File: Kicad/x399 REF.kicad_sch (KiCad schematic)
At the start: 75 parts, among them J1 +15V, J2 10Vref, Q1 MMBT3904, Q2 2SD882, Q3 AON7410, U1 LM399, U2 OP07

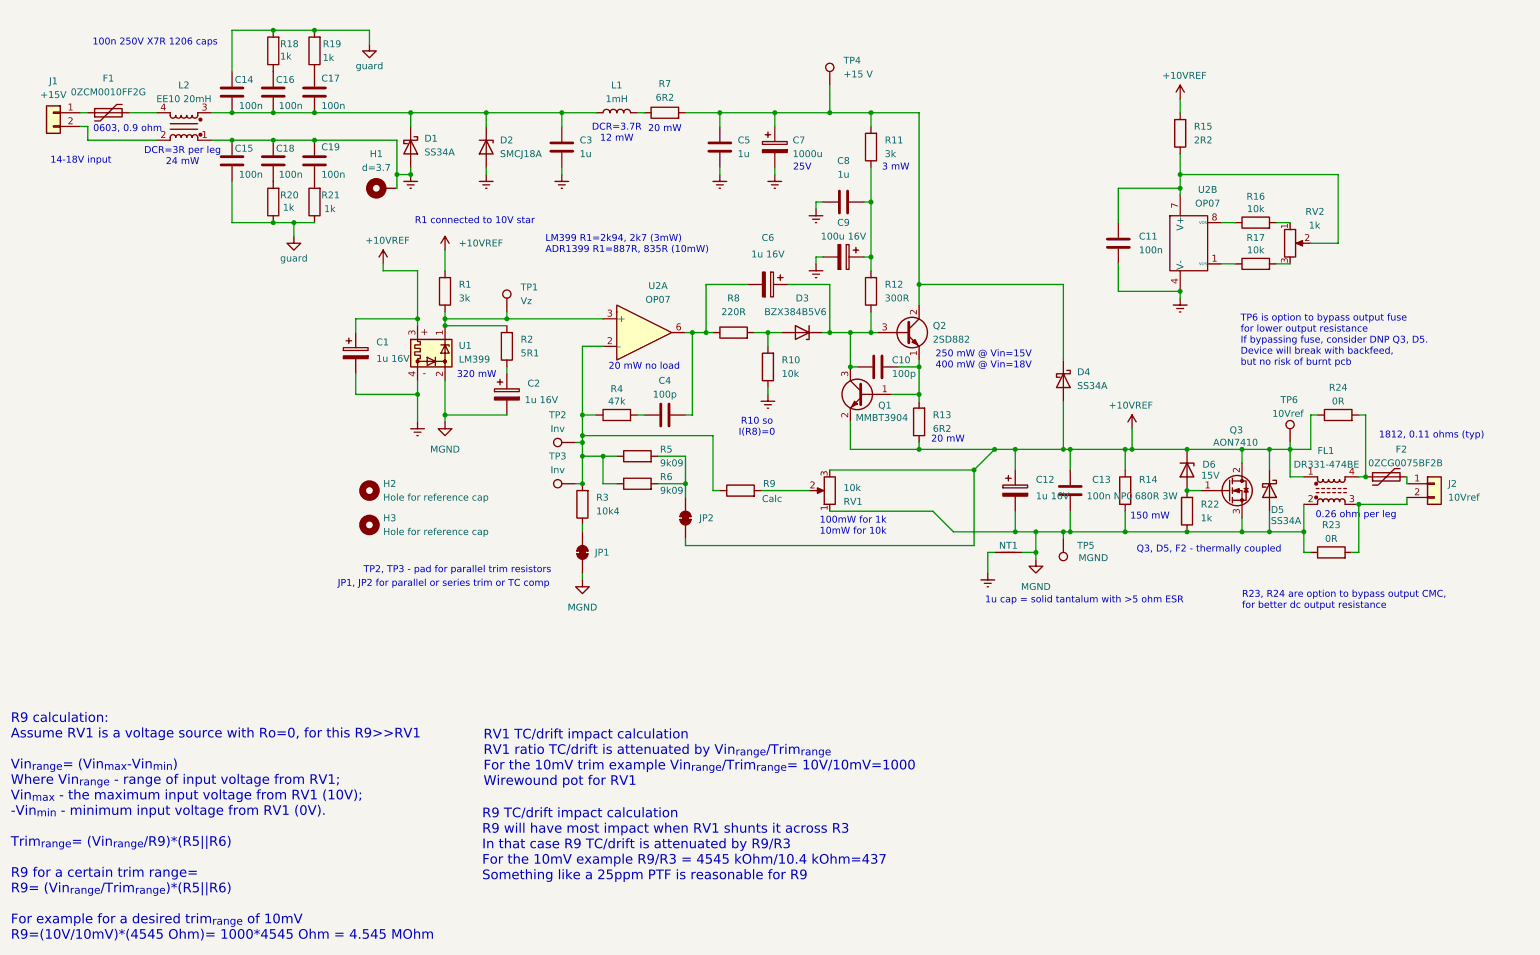
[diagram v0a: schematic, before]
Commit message: Add files via upload
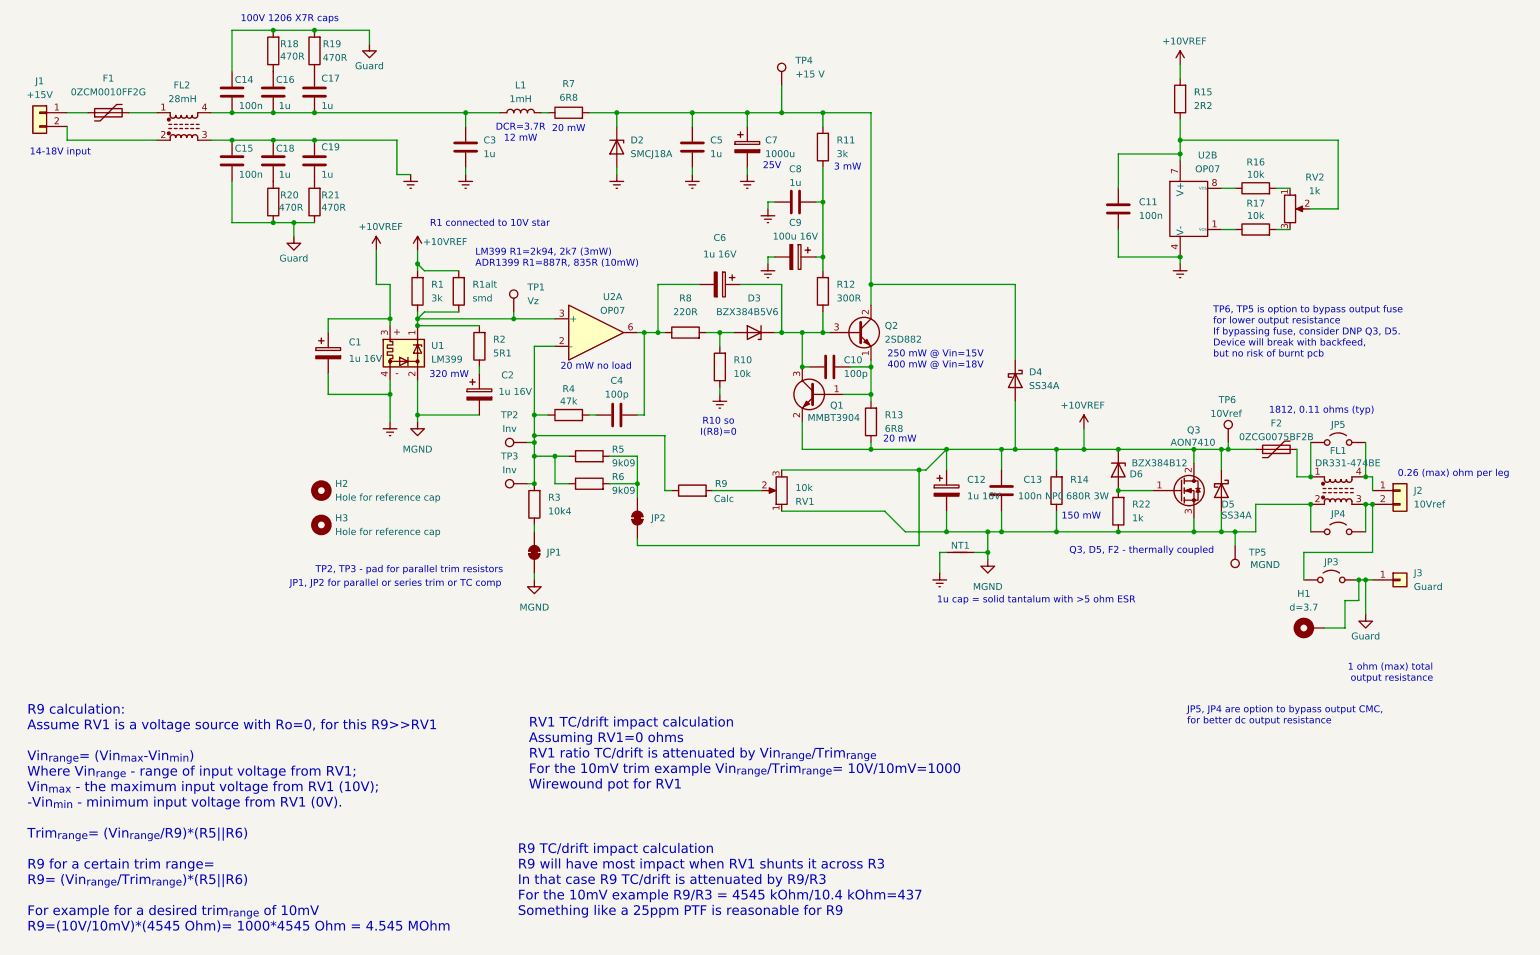
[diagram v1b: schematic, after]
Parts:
- removed D1: SS34A, Diode_SMD:D_SMA_Handsoldering, symbol Device:D_Schottky
- removed L2: EE10 20mH, symbol Device:Filter_EMI_CommonMode
- removed R23, R24: 0R, symbol Device:R
- added FL2: 28mH, OwnStuff:Universal line filter, symbol Filter:Choke_CommonMode_FerriteCore_1423
- added J3: Guard, Connector_Wire:SolderWire-0.127sqmm_1x01_D0.48mm_OD1mm_Relief, symbol Connector_Generic:Conn_01x01
- added JP3, JP4, JP5: ~, TestPoint:TestPoint_2Pads_Pitch2.54mm_Drill0.8mm, symbol Jumper:Jumper_2_Open
- added R1alt: smd, Resistor_SMD:R_1206_3216Metric_Pad1.30x1.75mm_HandSolder, symbol Device:R
- C16, C17, C18, C19: value 100n -> 1u; footprint Capacitor_SMD:C_0805_2012Metric_Pad1.18x1.45mm_HandSolder -> Capacitor_SMD:C_1206_3216Metric_Pad1.33x1.80mm_HandSolder
- D6: value 15V -> BZX384B12
- F2: footprint Resistor_SMD:R_0603_1608Metric_Pad0.98x0.95mm_HandSolder -> Resistor_SMD:R_1812_4532Metric_Pad1.30x3.40mm_HandSolder
- FL1: footprint (none) -> OwnStuff:L_CommonMode_Bourns_DR331_Handsolder
- JP1, JP2: footprint Jumper:Joined holes D=1.8 Dh=0.9 P=3mm -> OwnStuff:Joined holes D=1.8 Dh=0.9 P=3mm
- L1: footprint Inductor_SMD:L_7.3x7.3_H4.5_Handsoldering -> OwnStuff:L_7.3x7.3_H4.5_Handsoldering
- Q3: footprint (none) -> OwnStuff:AO DFN3x3 EP GDS
- R13, R7: value 6R2 -> 6R8
- R18, R19, R20, R21: value 1k -> 470R
- R3, R5, R6: footprint Resistor_THT:S5-61 -> OwnStuff:S5-61+vishay(150mil)+smd1206
- RV1, RV2: footprint Potentiometer_THT:Potentiometer_Soviet_SP5-2VB -> OwnStuff:Potentiometer_Soviet_SP5-2VB
- TP2, TP3: footprint TestPoint:TestPoint_THTPad_D1.8mm_Drill0.9mm -> OwnStuff:TestPoint_THTPad_D1.8mm_Drill0.9mm
- U1: footprint Package_TO_SOT_THT:Analog_TO-46-4_ThermalShield_balanced pins -> OwnStuff:Analog_TO-46-4_ThermalShield_balanced pins
- U2: footprint Package_DIP:DIP-8_W7.62mm_W_soic_under -> OwnStuff:DIP-8_W7.62mm_W_soic_under
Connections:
- net +10VREF: now also F2.1, R1alt.2; no longer FL1.1
- net Earth: now also FL2.3; no longer H1.1
- net MGND: now also JP4.1 (A)
- net at R1.1, R2.2, TP1.1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: now also R1alt.1
- net at C5.1, C7.1, D4.1 (K)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: now also D2.1 (K)
- net at J2.1 (Pin_1): now also FL1.4, JP5.2 (B); no longer F2.2
- net at FL1.3, J2.2 (Pin_2): now also JP3.1 (A), JP4.2 (B)
- net at C14.2, C16.2, C17.2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: now also FL2.4; no longer D2.1 (K)
- net at F1.2: now also FL2.1
- net at J1.2 (Pin_2): now also FL2.2
- net guard renamed Guard
- net Guard: now also H1.1, J3.1 (Pin_1), JP3.2 (B)
- new net: F2.2, FL1.1, JP5.1 (A)
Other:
- note added: "0.26 (max) ohm per leg"
- note added: "1 ohm (max) total output resistance"
- note added: "100V 1206 X7R caps"
- note added: "JP5, JP4 are option to bypass output CMC, for better dc output resistance"
- note added: "RV1 TC/drift impact calculation Assuming RV1=0 ohms RV1 ratio TC/drift is attenuated by Vin_{range}/Trim_{range} For the 10mV trim example Vin_{range}/Trim_{range}= 10V/10mV=1000 Wirewound pot for RV1"
- note added: "TP6, TP5 is option to bypass output fuse for lower output resistance If bypassing fuse, consider DNP Q3, D5. Device will break with backfeed, but no risk of burnt pcb"
- note removed: "0.26 ohm per leg"
- note removed: "0603, 0.9 ohm"
- note removed: "100mW for 1k 10mW for 10k"
- note removed: "100n 250V X7R 1206 caps"
- note removed: "DCR=3R per leg 24 mW"
- note removed: "R23, R24 are option to bypass output CMC, for better dc output resistance"
- note removed: "RV1 TC/drift impact calculation RV1 ratio TC/drift is attenuated by Vin_{range}/Trim_{range} For the 10mV trim example Vin_{range}/Trim_{range}= 10V/10mV=1000 Wirewound pot for RV1"
- note removed: "TP6 is option to bypass output fuse for lower output resistance If bypassing fuse, consider DNP Q3, D5. Device will break with backfeed, but no risk of burnt pcb"
- moved on the sheet: C1, C10, C11, C12, C13, C2, C3, C4, C5, C6, C7, C8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
